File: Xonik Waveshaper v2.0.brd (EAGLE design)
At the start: 63.5 x 28.8 mm, 89 parts, among them IC1 TL074D, IC2 TL074D, IC3 TL074D, IC4 TL072D, IC5 4013D, T1 2n3904

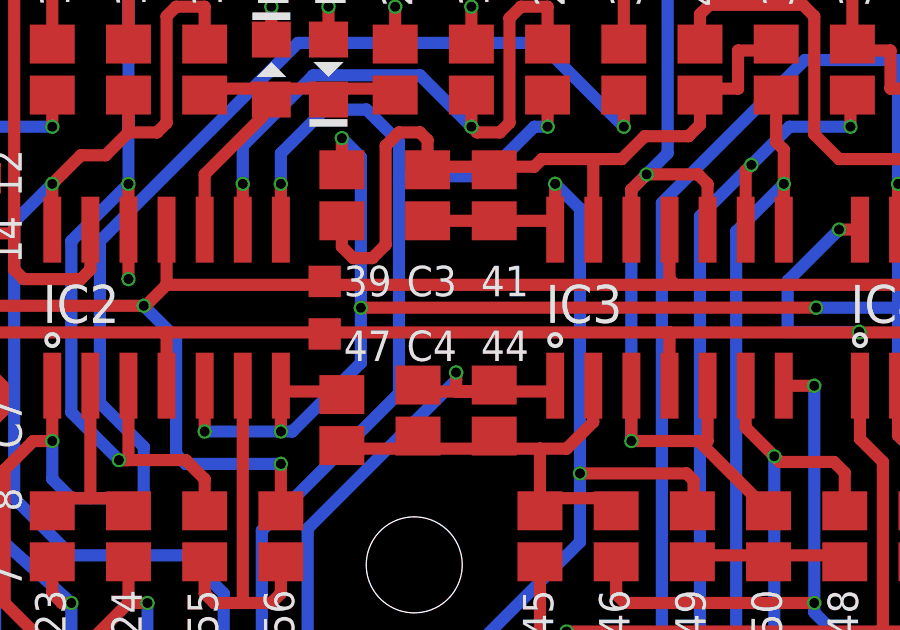
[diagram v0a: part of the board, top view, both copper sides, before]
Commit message: Silk screen tweak
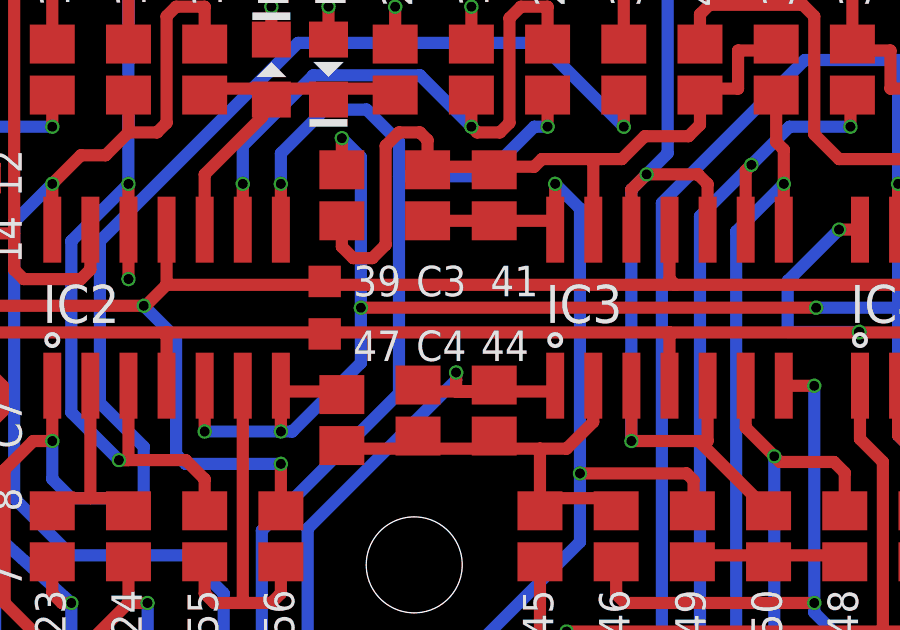
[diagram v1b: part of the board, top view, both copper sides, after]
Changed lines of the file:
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@@
 <text x="46.9265" y="26.543" size="1.016" layer="25" rot="R90">37</text>
 <text x="44.3865" y="26.543" size="1.016" layer="25" rot="R90">38</text>
-<text x="29.4005" y="16.891" size="1.016" layer="25">39</text>
+<text x="29.718" y="16.891" size="1.016" layer="25">39</text>
 <text x="41.8465" y="26.543" size="1.016" layer="25" rot="R90">40</text>
-<text x="33.9725" y="16.891" size="1.016" layer="25">41</text>
+<text x="34.29" y="16.891" size="1.016" layer="25">41</text>
 <text x="33.9725" y="14.732" size="1.016" layer="25">44</text>
 <text x="35.3695" y="7.112" size="1.016" layer="25" rot="R270">45</text>
 <text x="37.9095" y="7.112" size="1.016" layer="25" rot="R270">46</text>
-<text x="29.4005" y="14.732" size="1.016" layer="25">47</text>
+<text x="29.718" y="14.732" size="1.016" layer="25">47</text>
 <text x="45.5295" y="7.112" size="1.016" layer="25" rot="R270">48</text>
 <text x="40.4495" y="7.112" size="1.016" layer="25" rot="R270">49</text>
@@
 <text x="48.0695" y="7.239" size="1.016" layer="25" rot="R270">C1</text>
 <text x="54.5465" y="26.416" size="1.016" layer="25" rot="R90">C2</text>
-<text x="31.496" y="16.891" size="1.016" layer="25">C3</text>
-<text x="31.496" y="14.732" size="1.016" layer="25">C4</text>
+<text x="31.8135" y="16.891" size="1.016" layer="25">C3</text>
+<text x="31.8135" y="14.732" size="1.016" layer="25">C4</text>
 <text x="62.1665" y="26.416" size="1.016" layer="25" rot="R90">C5</text>
 <text x="58.42" y="7.112" size="1.016" layer="25" rot="R270">C6</text>
